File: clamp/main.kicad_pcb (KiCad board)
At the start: 2 copper layers, 37 parts, among them P1 CONN_01X12, U1 LM741, U2 LM741, U3 LM741, U4 LM741, U5 LM741, U6 LM741

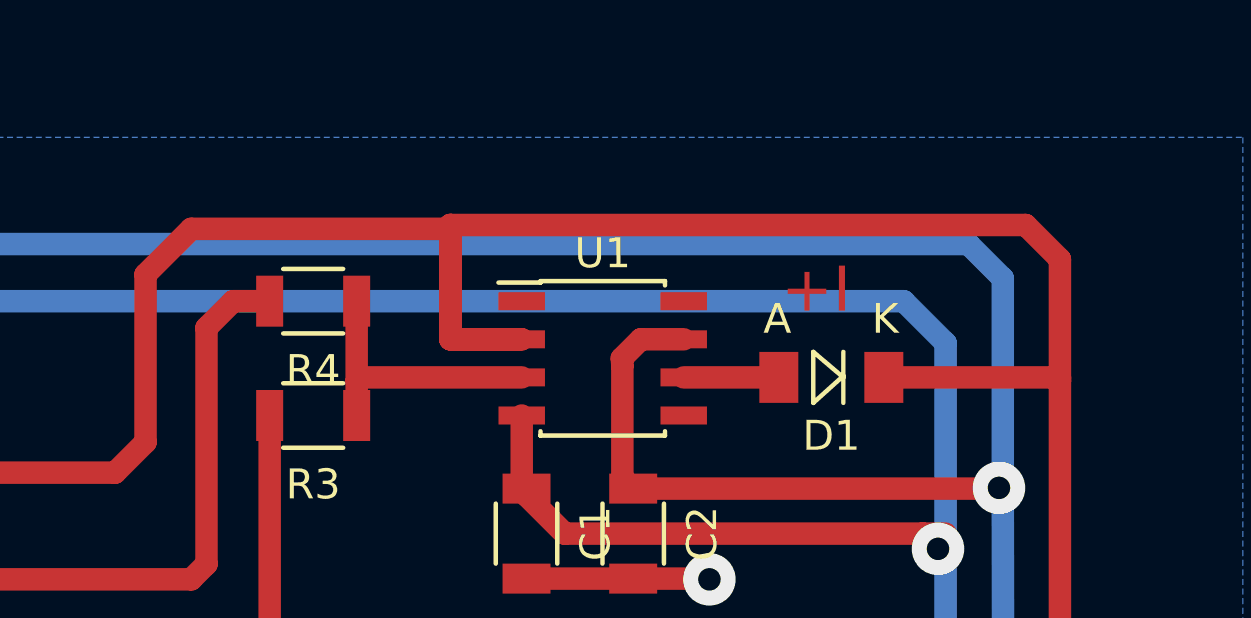
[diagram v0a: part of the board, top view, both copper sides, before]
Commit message: tidy
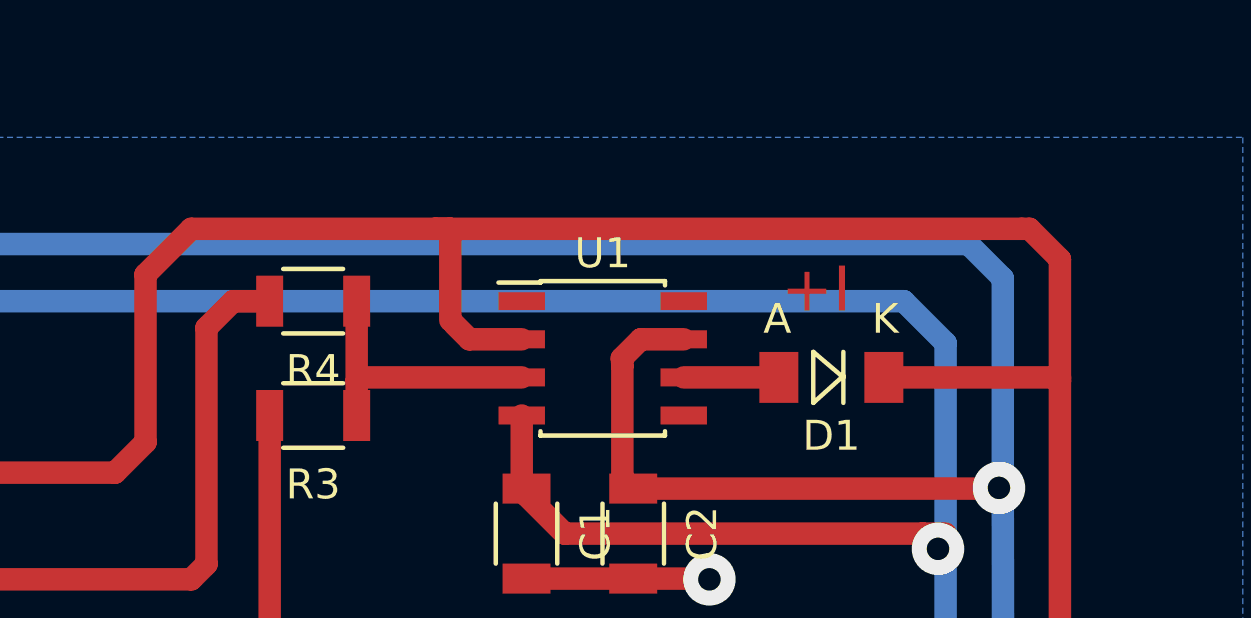
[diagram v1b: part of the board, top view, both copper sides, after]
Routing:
- net OUT: track 223.4 -> 216.8 mm
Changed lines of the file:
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@@
     (thickness 1.6)
     (drawings 13)
-    (tracks 343)
+    (tracks 341)
     (zones 0)
     (modules 37)
@@
   (segment (start 157.988 132.588) (end 157.861 132.588) (width 0.75) (layer B.Cu) (net 4))
   (via (at 157.988 132.588) (size 1.75) (drill 0.75) (layers F.Cu B.Cu) (net 4))
+  (segment (start 149.352 85.852) (end 149.352 88.9) (width 0.75) (layer F.Cu) (net 5))
+  (segment (start 149.987 89.535) (end 151.732 89.535) (width 0.75) (layer F.Cu) (net 5))
+  (segment (start 149.479 89.027) (end 149.987 89.535) (width 0.75) (layer F.Cu) (net 5))
+  (segment (start 168.402 85.852) (end 168.656 85.852) (width 0.75) (layer F.Cu) (net 5))
+  (segment (start 168.656 85.852) (end 169.672 86.868) (width 0.75) (layer F.Cu) (net 5))
+  (segment (start 168.402 85.852) (end 149.352 85.852) (width 0.75) (layer F.Cu) (net 5))
+  (segment (start 169.672 90.932) (end 169.672 86.868) (width 0.75) (layer F.Cu) (net 5))
+  (segment (start 149.352 85.852) (end 148.844 85.852) (width 0.75) (layer F.Cu) (net 5))
   (segment (start 169.672 135.128) (end 169.672 138.684) (width 0.75) (layer F.Cu) (net 5))
   (segment (start 168.656 139.7) (end 163.80206 139.7) (width 0.75) (layer F.Cu) (net 5) (status 20))
@@
   (segment (start 149.733 103.505) (end 149.352 103.124) (width 0.75) (layer F.Cu) (net 5))
   (segment (start 139.192 87.376) (end 140.716 85.852) (width 0.75) (layer F.Cu) (net 5))
-  (segment (start 140.716 85.852) (end 149.352 85.852) (width 0.75) (layer F.Cu) (net 5))
-  (segment (start 149.352 85.852) (end 149.352 85.725) (width 0.75) (layer F.Cu) (net 5))
+  (segment (start 126.492 93.98) (end 138.176 93.98) (width 0.75) (layer F.Cu) (net 5))
+  (segment (start 138.176 93.98) (end 139.192 92.964) (width 0.75) (layer F.Cu) (net 5))
   (segment (start 139.192 92.964) (end 139.192 87.376) (width 0.75) (layer F.Cu) (net 5))
-  (segment (start 138.176 93.98) (end 139.192 92.964) (width 0.75) (layer F.Cu) (net 5))
+  (segment (start 140.716 85.852) (end 148.844 85.852) (width 0.75) (layer F.Cu) (net 5))
+  (segment (start 148.844 85.852) (end 149.352 85.852) (width 0.75) (layer F.Cu) (net 5))
   (segment (start 118.11 93.98) (end 126.492 93.98) (width 0.75) (layer F.Cu) (net 5) (status 10))
-  (segment (start 126.492 93.98) (end 138.176 93.98) (width 0.75) (layer F.Cu) (net 5))
   (segment (start 125.402 96.52) (end 125.476 96.52) (width 0.75) (layer F.Cu) (net 5) (status 30))
-  (segment (start 151.732 89.535) (end 149.479 89.535) (width 0.75) (layer F.Cu) (net 5) (status 10))
-  (segment (start 149.479 89.535) (end 149.352 89.408) (width 0.75) (layer F.Cu) (net 5))
-  (segment (start 149.352 89.408) (end 149.352 85.725) (width 0.75) (layer F.Cu) (net 5))
-  (segment (start 149.352 89.408) (end 149.352 85.725) (width 0.75) (layer F.Cu) (net 5))
   (segment (start 150.368 124.46) (end 149.86 123.952) (width 0.75) (layer F.Cu) (net 5))
   (segment (start 163.068 120.904) (end 150.368 120.904) (width 0.75) (layer F.Cu) (net 5))
@@
   (segment (start 169.672 135.128) (end 150.368 135.128) (width 0.75) (layer F.Cu) (net 5))
   (segment (start 150.368 135.128) (end 149.781846 135.518769) (width 0.75) (layer F.Cu) (net 5))
-  (segment (start 149.352 89.535) (end 149.352 89.408) (width 0.75) (layer F.Cu) (net 5))
-  (segment (start 149.352 89.408) (end 149.352 89.535) (width 0.75) (layer F.Cu) (net 5))
   (segment (start 163.80206 104.648) (end 169.672 104.648) (width 0.75) (layer F.Cu) (net 5) (status 10))
   (segment (start 163.80206 125.476) (end 169.672 125.476) (width 0.75) (layer F.Cu) (net 5) (status 10))
   (segment (start 163.80206 90.805) (end 169.672 90.805) (width 0.75) (layer F.Cu) (net 5) (status 10))
   (segment (start 169.672 90.805) (end 169.672 90.932) (width 0.75) (layer F.Cu) (net 5))
-  (segment (start 149.352 85.725) (end 168.529 85.725) (width 0.75) (layer F.Cu) (net 5))
-  (segment (start 169.672 86.868) (end 169.672 90.932) (width 0.75) (layer F.Cu) (net 5))
-  (segment (start 168.529 85.725) (end 169.672 86.868) (width 0.75) (layer F.Cu) (net 5))
   (segment (start 169.672 125.476) (end 169.672 135.128) (width 0.75) (layer F.Cu) (net 5))
   (segment (start 169.672 90.932) (end 169.672 100.076) (width 0.75) (layer F.Cu) (net 5))
   (segment (start 169.672 100.076) (end 169.672 104.648) (width 0.75) (layer F.Cu) (net 5))
   (segment (start 169.672 104.648) (end 169.672 125.476) (width 0.75) (layer F.Cu) (net 5))
-  (segment (start 151.732 89.535) (end 149.352 89.535) (width 0.75) (layer F.Cu) (net 5) (status 10))
   (segment (start 157.132 104.775) (end 160.30194 104.648) (width 0.75) (layer F.Cu) (net 6) (status 30))
   (segment (start 122.502 96.52) (end 118.11 96.52) (width 0.75) (layer F.Cu) (net 7) (status 30))
